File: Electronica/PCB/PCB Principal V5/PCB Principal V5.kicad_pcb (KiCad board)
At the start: 2 copper layers, 139.1 x 70 mm, 19 parts, among them J1 Conexion Sensores, J12 TP, J2 Power Monster, J3 On/Off General, J4 Power Input 2, J5 IDC Placa Botones, J6 Power Input 1, SW1 On/Off Motores

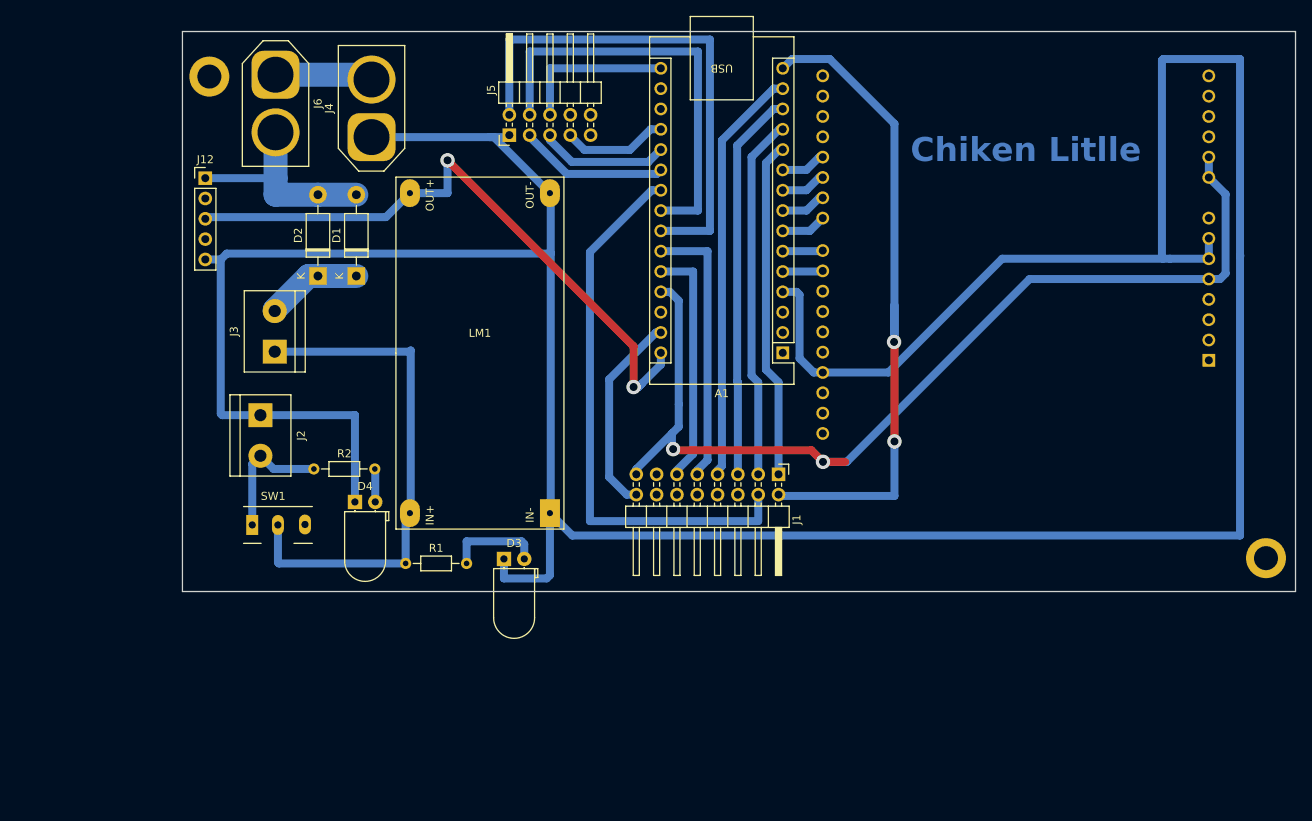
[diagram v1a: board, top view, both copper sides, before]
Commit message: PCB V5 LINDA HERMOSA DIVINA
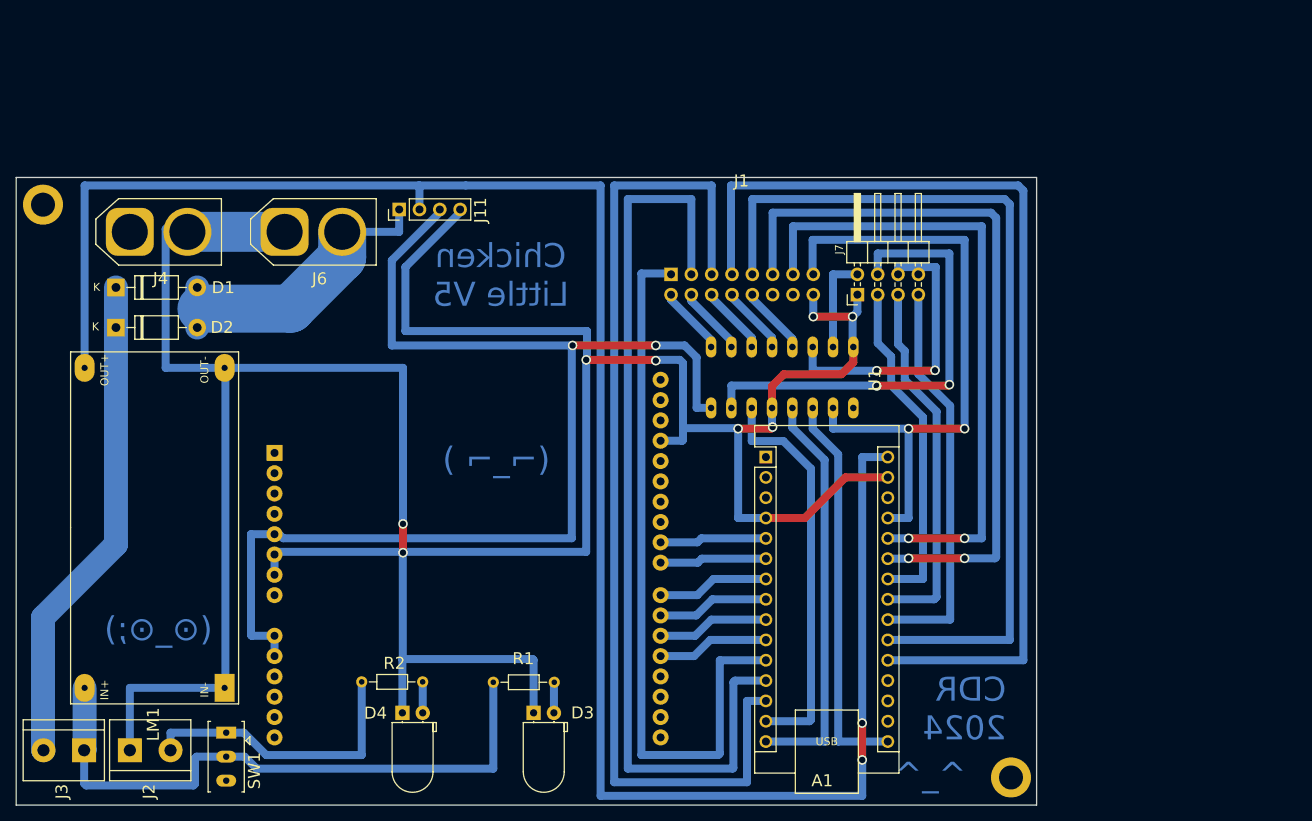
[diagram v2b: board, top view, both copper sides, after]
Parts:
- removed the ? at (261.9, 91.2)
- removed the ? at (129.8, 31.0)
- removed J12: TP, Connector_PinHeader_2.54mm:PinHeader_1x05_P2.54mm_Vertical
- removed J5: IDC Placa Botones, Connector_PinHeader_2.54mm:PinHeader_2x05_P2.54mm_Horizontal
- added ?: , , F.Cu at (109.0, 47.0)
- added ?: , , F.Cu at (230.0, 118.6)
- added J11: Conn_01x04_Pin, Connector_PinHeader_2.54mm:PinHeader_1x04_P2.54mm_Vertical, F.Cu at (153.5, 47.6)
- added J7: Placa de Botones, Connector_PinHeader_2.54mm:PinHeader_2x04_P2.54mm_Horizontal, F.Cu at (210.8, 58.2)
- added U1: 74HC595, 74HC595N_DIP16_:DIP16-2.54-20.32X5.84MM, B.Cu at (201.4, 68.6)
- J1: moved to B.Cu
- LM1: footprint Step Down:LM2596_correctedMeas -> StepDown:StepDown
- SW1: footprint Button_Switch_THT:SW_Slide_SPDT_Angled_CK_OS102011MA1Q -> Button_Switch_THT:SW_Slide_SPDT_Straight_CK_OS102011MS2Q
- moved A2 117.4 mm to (137.9, 78.0), turned to -90 degrees
- moved J3 55.2 mm to (114.1, 115.2), turned to 180 degrees
- moved LM1 46.2 mm to (123.0, 87.4)
- moved J2 45.0 mm to (119.9, 115.2), turned to 0 degrees
- moved J4 32.5 mm to (119.9, 50.4), turned to 0 degrees
- moved D1 30.1 mm to (118.1, 57.4), turned to 0 degrees
- moved J1 28.4 mm to (187.5, 55.7)
- moved SW1 27.3 mm to (131.9, 114.0), turned to -90 degrees
- moved R2 27.3 mm to (148.8, 106.7)
- moved D4 27.0 mm to (153.9, 110.5)
- moved D2 26.1 mm to (118.1, 62.4), turned to 0 degrees
- moved J6 19.7 mm to (139.2, 50.4), turned to 0 degrees
- moved D3 19.6 mm to (170.3, 110.5)
- moved R1 18.5 mm to (165.3, 106.7)
- moved A1 13.2 mm to (199.4, 78.5), turned to 0 degrees
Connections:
- A1 pad 11: TRIG 2 -> ECHO 1
- A1 pad 13: TRIG 1 -> ECHO 3
- A1 pad 14: ECHO 1 -> Data
- A1 pad 15: ECHO 3 -> Latch
- A1 pad 16: LED4 -> Clock
- A1 pad 19: LED1 -> unconnected-(A1-A0-Pad19)
- A1 pad 20: BTN1 -> ECHO 4
- A1 pad 21: BTN2 -> ECHO 5
- A1 pad 22: TRIG 3 -> LED1
- A1 pad 23: LED3 -> BTN1
- A1 pad 24: LED2 -> BTN2
- A1 pad 25: CNY 1 -> CNY 2
- A1 pad 26: CNY 2 -> CNY 1
- J1 pad 1: TRIG 2 -> ECHO 1
- J1 pad 10: TRIG 4 -> TRIG 1
- J1 pad 12: ECHO 5 -> unconnected-(J1-Pin_12-Pad12)
- J1 pad 13: CNY 3 -> CNY 1
- J1 pad 14: TRIG 5 -> unconnected-(J1-Pin_14-Pad14)
- J1 pad 2: ECHO 3 -> TRIG 2
- J1 pad 5: TRIG 1 -> ECHO 3
- J1 pad 6: unconnected-(J1-Pin_6-Pad6) -> TRIG 5
- J1 pad 7: ECHO 1 -> ECHO 4
- J1 pad 8: ECHO 4 -> TRIG 4
- J1 pad 9: CNY 1 -> ECHO 5
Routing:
- net VNano: track 81.0 -> 244.9 mm
- net ECHO 4: track 0.00 -> 123.6 mm
- net ECHO 5: track 0.00 -> 111.6 mm
- net +5V: track 126.3 -> 228.7 mm, vias 2 -> 4
- net ECHO 2: track 45.3 -> 116.2 mm
- net GND: track 453.3 -> 385.7 mm, vias 0 -> 8
- net CNY 2: track 30.2 -> 92.0 mm, vias 0 -> 2
- net TRIG 3: track 70.0 -> 8.61 mm
- net LED2: track 64.5 -> 12.2 mm
- net Latch: track 0.00 -> 50.7 mm
- net Data: track 0.00 -> 50.1 mm
- net Net-(D1-K): track 12.1 -> 61.7 mm
- net Clock: track 0.00 -> 49.2 mm
- net CNY 1: track 34.3 -> 80.4 mm, vias 0 -> 2
- net ECHO 3: track 83.5 -> 127.0 mm, vias 2 -> 0
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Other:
- board size 139.1 x 70 mm -> 127.5 x 78.4 mm
- board text added: "(¬_¬ )"
- board text added: "(⊙_⊙;)"
- board text added: "CDR 2024"
- board text added: "Chicken Little V5"
- board text added: "^_^"
- board text removed: "Chiken Litlle"
